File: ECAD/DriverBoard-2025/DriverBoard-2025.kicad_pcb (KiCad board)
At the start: 2 copper layers, 56 x 45 mm, 23 parts, among them J1 XT30, J2 Conn_01x04, J3 Conn_01x04, J4 Conn_01x04, J5 Fan, SW1 SW_DIP_x02, U1 TMC2209_SILENTSTEPSTICK, U2 TMC2209_SILENTSTEPSTICK, U3 TMC2209_SILENTSTEPSTICK

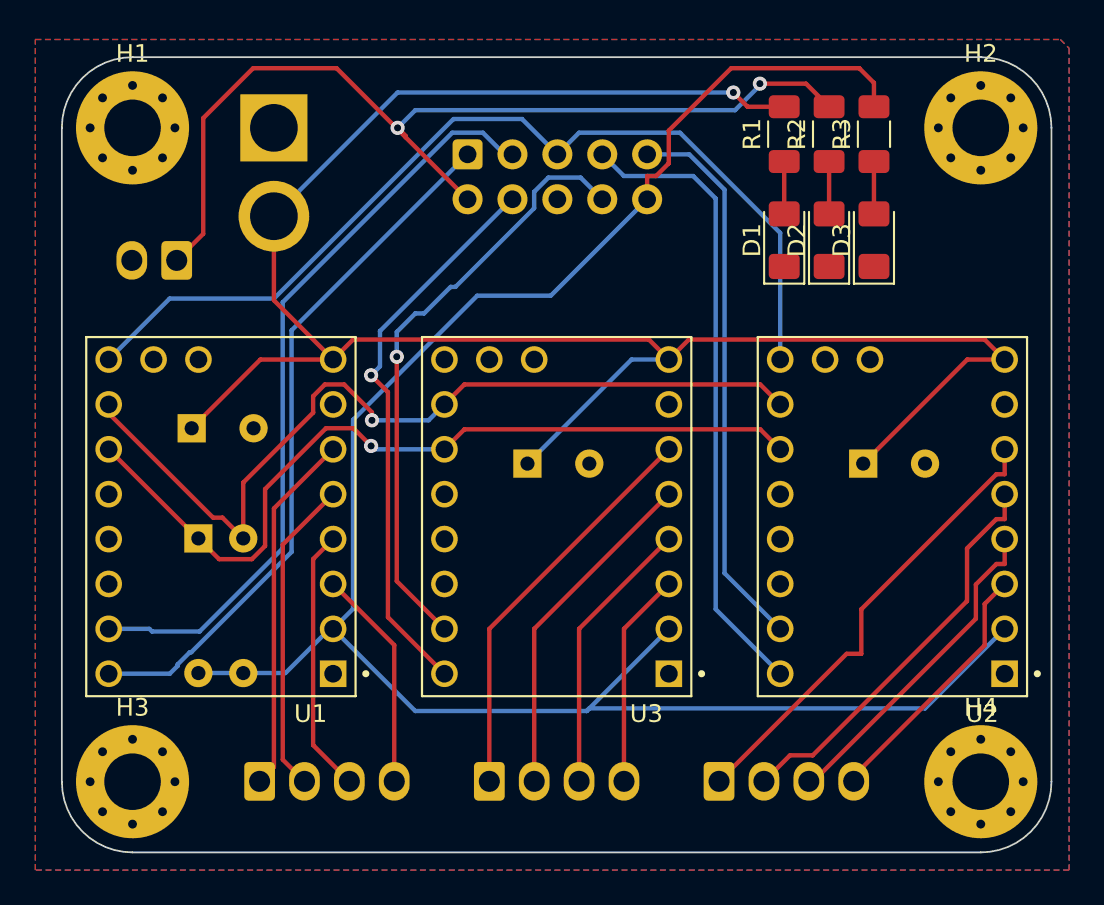
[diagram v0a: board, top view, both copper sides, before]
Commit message: PCB routing completed
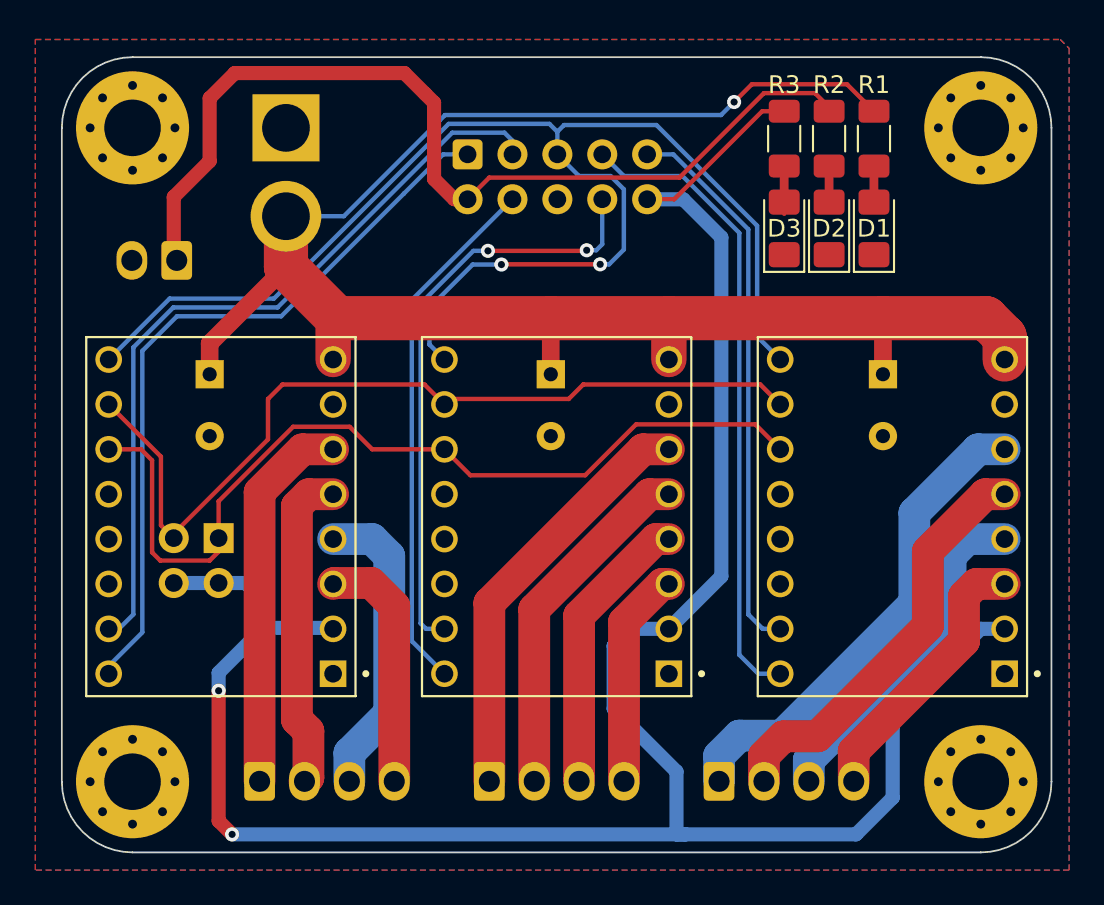
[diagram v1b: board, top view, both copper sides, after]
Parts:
- SW1: footprint Button_Switch_THT:SW_DIP_SPSTx02_Slide_9.78x7.26mm_W7.62mm_P2.54mm -> Connector_PinHeader_2.54mm:PinHeader_2x02_P2.54mm_Vertical
- moved C2 5.23 mm to (137.7, 67.9), turned to -90 degrees
- moved C3 5.18 mm to (156.5, 67.9), turned to -90 degrees
- moved D1 5.12 mm to (156.0, 59.7)
- moved D3 5.12 mm to (150.9, 59.7)
- moved R1 5.09 mm to (156.0, 54.6)
- moved R3 5.09 mm to (150.9, 54.6)
- moved C1 3.22 mm to (118.4, 67.9), turned to -90 degrees
- moved SW1 1.15 mm to (118.9, 77.2), turned to 180 degrees
- moved J1 0.68 mm to (122.7, 54.0)
- moved D2 0.67 mm to (153.4, 59.7)
- moved R2 0.25 mm to (153.4, 54.6)
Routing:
- net EN: track 54.5 -> 78.0 mm, vias 0 -> 2
- net +3V3: track 110.7 -> 129.8 mm, vias 0 -> 2
- net +24V: track 112.0 -> 102.6 mm
- net MS2: track 47.0 -> 51.4 mm, vias 1 -> 0
- net Net-(J2-Pin_3): track 15.0 -> 17.3 mm
- net DIR_1: track 39.9 -> 42.1 mm
- net STEP_3: track 31.9 -> 30.0 mm, vias 1 -> 0
- net Net-(J3-Pin_1): track 26.2 -> 27.8 mm
- net Net-(J2-Pin_4): track 12.6 -> 13.9 mm
- net STEP_1: track 43.3 -> 44.3 mm
- net Net-(J2-Pin_1): track 20.5 -> 21.5 mm
- net Net-(J3-Pin_4): track 14.7 -> 15.6 mm
- net Net-(D2-A): track 2.96 -> 2.04 mm
- net Net-(D1-A): track 2.96 -> 2.04 mm
- net Net-(D3-A): track 2.96 -> 2.04 mm
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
